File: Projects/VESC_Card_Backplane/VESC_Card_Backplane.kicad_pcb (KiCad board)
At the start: 2 copper layers, 40 parts, among them M1 FE1.1S, P1 USB_OTG, P10 AMP17614426-2_EDGE, P11 CONN_01X06, P2 EC90_Flat, P3 AMP17614426-2_EDGE, P4 CONN_01X06, P5 CONN_01X04, P5V1 CONN_01X02, P6 EC90_Flat, P7 AMP17614426-2_EDGE, P8 CONN_01X06, P9 EC90_Flat, U1 LP38693

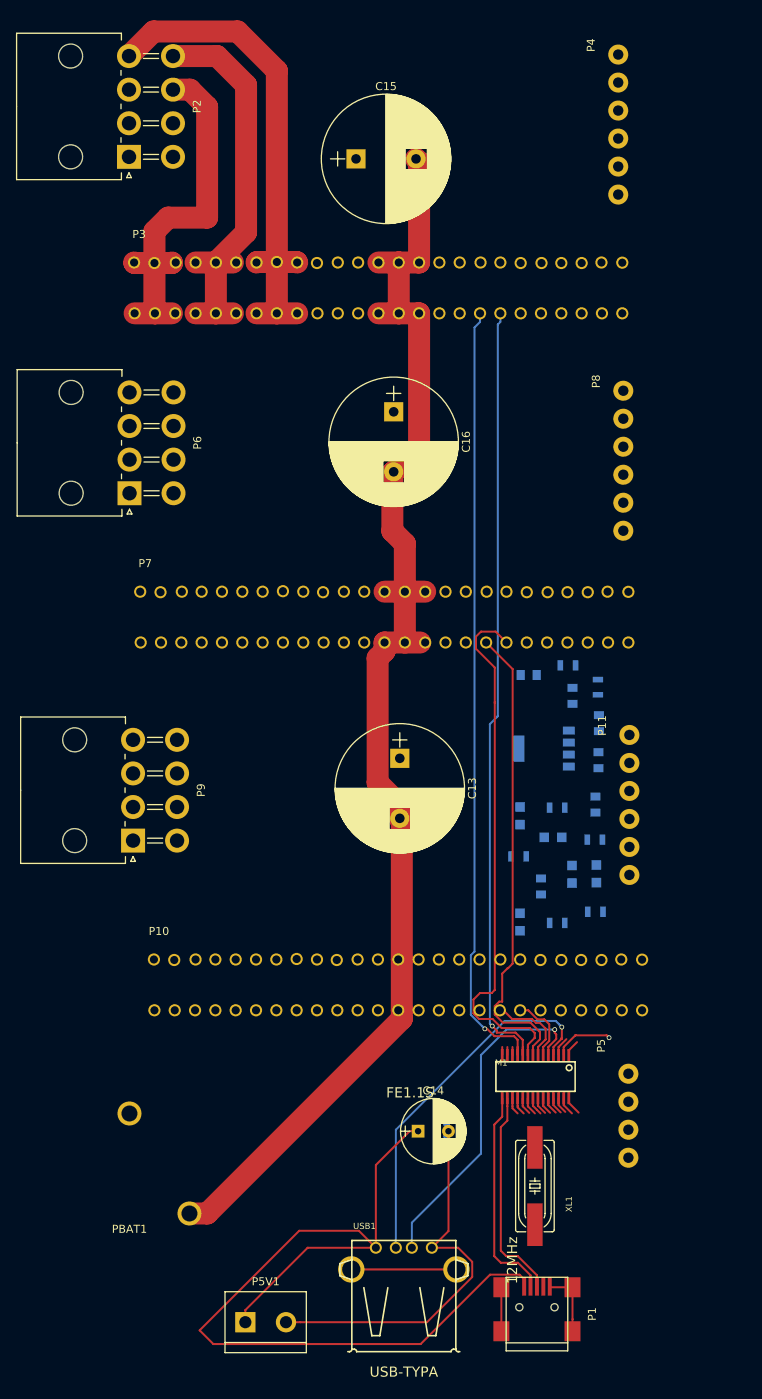
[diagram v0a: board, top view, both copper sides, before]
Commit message: Comleted VESC Backplane
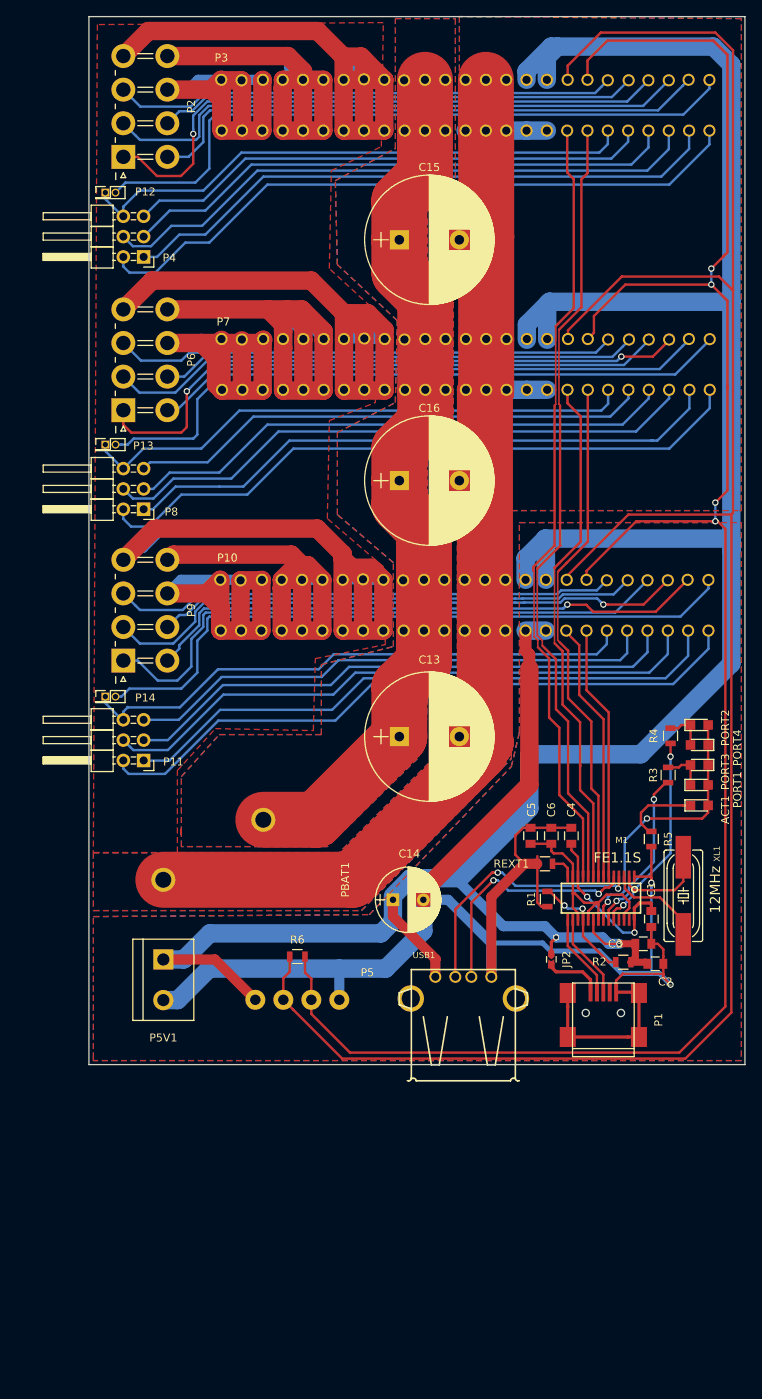
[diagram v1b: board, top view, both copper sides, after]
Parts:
- removed JP1: Jumper_NC_Small, USST-footprints:J_0603
- removed U1: LP38693, USST-footprints:SOT-223_5-pin
- added JP2: J, USST-footprints:J_0603, F.Cu at (86.0, 132.4)
- added P12: CONN_01X02, Pin_Headers:Pin_Header_Straight_2x01_Pitch1.27mm, F.Cu at (30.2, 36.6)
- added P13: CONN_01X02, Pin_Headers:Pin_Header_Straight_2x01_Pitch1.27mm, F.Cu at (30.2, 68.1)
- added P14: CONN_01X02, Pin_Headers:Pin_Header_Straight_2x01_Pitch1.27mm, F.Cu at (30.2, 99.6)
- ACT1, C1, C2, C3, C4, C5, C6, PORT1, PORT2, PORT3, PORT4, R1, R2, R3, R4, R5, R6, REXT1: moved to F.Cu
- P11, P4, P8: footprint USST-footprints:Molex_39502_1006R -> Pin_Headers:Pin_Header_Angled_2x03_Pitch2.54mm
- P2, P6, P9: footprint Connectors_Molex:Molex_MiniFit-JR-5569-08A2_2x04x4.20mm_Angled -> USST-footprints:Molex_MiniFit-JR-5569-08A2_2x04x4.20mm_Angled_Overhang
- moved P11 62.4 mm to (35.0, 107.6), turned to 180 degrees
- moved P8 60.0 mm to (35.0, 76.2), turned to 180 degrees
- moved P4 59.8 mm to (35.0, 44.6), turned to 180 degrees
- moved P5 50.6 mm to (49.0, 137.5), turned to 0 degrees
- moved R6 49.7 mm to (54.2, 132.1)
- moved P10 48.2 mm to (80.2, 99.0)
- moved P5V1 44.7 mm to (37.5, 135.0), turned to 270 degrees
- moved XL1 40.8 mm to (102.5, 124.5), turned to 90 degrees
- moved P1 37.7 mm to (92.5, 140.0)
- moved USB1 34.7 mm to (75.0, 140.0)
- moved P7 33.2 mm to (80.4, 68.9)
- moved C1 29.6 mm to (98.5, 127.4)
- moved PBAT1 29.5 mm to (37.5, 122.5), turned to 90 degrees
- moved C14 29.1 mm to (66.2, 125.0)
- moved ACT1 26.7 mm to (104.5, 113.2), turned to 0 degrees
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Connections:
- M1 pad 25: Net-(M1-Pad25) -> (no net)
- M1 pad 27: Net-(M1-Pad27) -> (no net)
- M1 pad 8: /USB_DP_2 -> /USB_DM_2
- M1 pad 9: /USB_DM_2 -> /USB_DP_2
- P1 pad 1: +5V -> Net-(JP2-Pad2)
- P1 pad 4: Net-(P1-Pad4) -> (no net)
- P1 pad 5: Net-(P1-Pad5) -> GND
- P1 pad 6: Net-(P1-Pad5) -> GND
- P10 pad 21: Net-(P10-Pad21) -> /Motor_Controller_C/GND_AUX
- P11 pad 1: Net-(P10-Pad21) -> Net-(P10-Pad17)
- P11 pad 2: Net-(P10-Pad20) -> Net-(P10-Pad16)
- P11 pad 5: Net-(P10-Pad17) -> Net-(P10-Pad20)
- P11 pad 6: Net-(P10-Pad16) -> /Motor_Controller_C/GND_AUX
- P3 pad 21: Net-(P3-Pad21) -> /Motor_Controller_A/GND_AUX
- P3 pad 24: GND -> /PGND
- P3 pad 25: GND -> /PGND
- P4 pad 1: Net-(P3-Pad21) -> Net-(P3-Pad17)
- P4 pad 2: Net-(P3-Pad20) -> Net-(P3-Pad16)
- P4 pad 5: Net-(P3-Pad17) -> Net-(P3-Pad20)
- P4 pad 6: Net-(P3-Pad16) -> /Motor_Controller_A/GND_AUX
- P7 pad 21: Net-(P7-Pad21) -> /Motor_Controller_B/GND_AUX
- P7 pad 24: GND -> /PGND
- P7 pad 25: GND -> /PGND
- P8 pad 1: Net-(P7-Pad21) -> Net-(P7-Pad17)
- P8 pad 2: Net-(P7-Pad20) -> Net-(P7-Pad16)
- P8 pad 5: Net-(P7-Pad17) -> Net-(P7-Pad20)
- P8 pad 6: Net-(P7-Pad16) -> /Motor_Controller_B/GND_AUX
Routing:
- net /CANH: track 0.00 -> 262.0 mm
- net /CAN_Bus/CANL: track 0.00 -> 247.3 mm, vias 0 -> 4
- net +5V: track 114.8 -> 346.6 mm, vias 0 -> 2
- net GND: track 50.8 -> 219.2 mm, vias 0 -> 2
- net /Motor_Controller_B/Y: track 0.00 -> 120.6 mm
- net /Motor_Controller_C/Y: track 0.00 -> 116.1 mm
- net /VBAT: track 0.00 -> 110.0 mm
- net /Motor_Controller_B/X: track 0.00 -> 86.6 mm
- net /Motor_Controller_C/X: track 0.00 -> 84.8 mm
- net Net-(P12-Pad2): track 0.00 -> 84.2 mm
- net Net-(P10-Pad15): track 0.00 -> 84.0 mm
- net Net-(P7-Pad16): track 0.00 -> 83.3 mm
- net Net-(P10-Pad16): track 0.00 -> 83.2 mm
- net Net-(P3-Pad16): track 0.00 -> 83.1 mm
- net Net-(P13-Pad2): track 0.00 -> 82.3 mm
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- added copper zone on B.Cu, net /PGND
- added copper zone on F.Cu, net /PGND
- added copper zone on B.Cu, net /VBAT
- added copper zone on F.Cu, net /VBAT
- added copper zone on B.Cu, net GND
- added copper zone on F.Cu, net GND
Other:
- board outline added: 82 x 131 mm
- net class Default: trace_width 0.25 -> 0.2032; via_dia 0.6 -> 0.508; via_drill 0.4 -> 0.254
- rule trace_min: 0.2 -> 0.2032
- rule via_min_drill: 0.3 -> 0.254
- rule via_min_size: 0.4 -> 0.508
